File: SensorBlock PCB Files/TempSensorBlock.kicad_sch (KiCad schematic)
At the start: 11 parts, among them J1 Source Input (Screw), J2 Microcontroller Terminal (Scr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, U1 LM75B

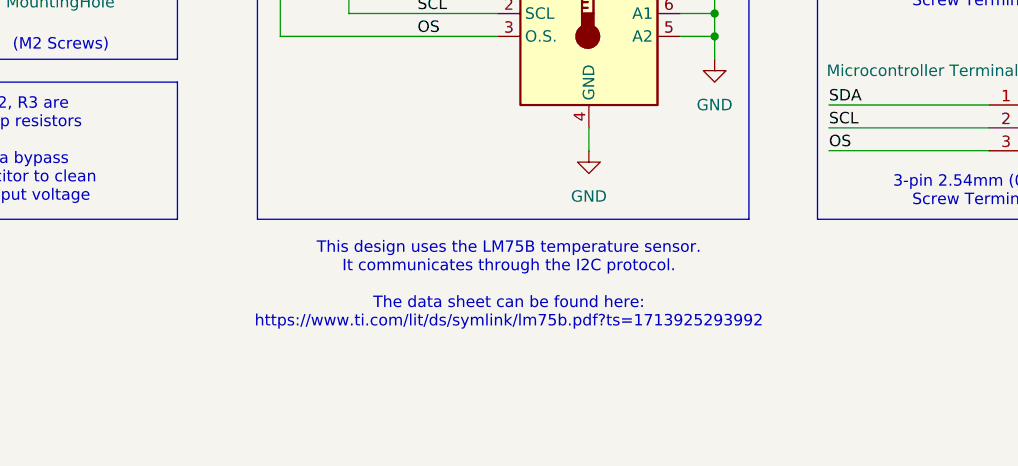
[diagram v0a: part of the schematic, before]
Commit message: Added documentation
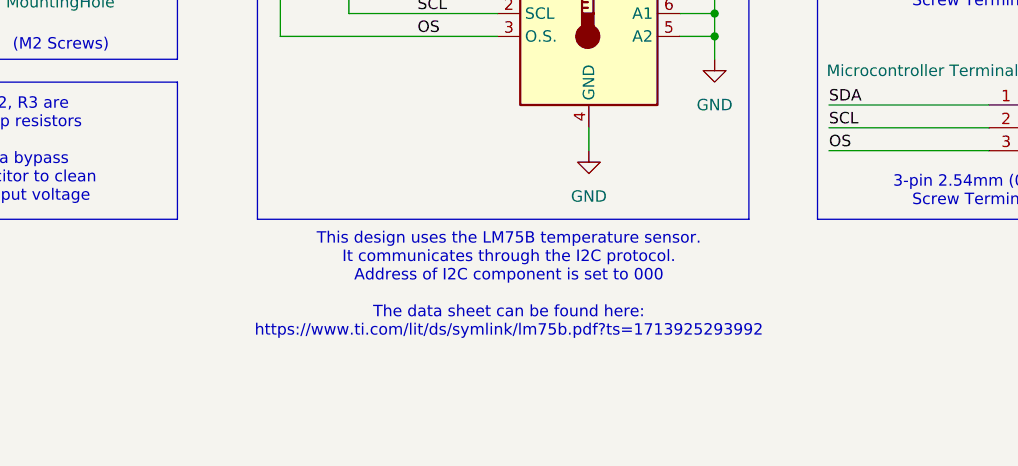
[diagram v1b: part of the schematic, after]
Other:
- note added: "This design uses the LM75B temperature sensor. It communicates through the I2C protocol. Address of I2C component is set to 000 The data sheet can be found here: https://www.ti.com/lit/ds/symlink/lm75b.pdf?ts=1713925293992"
- note removed: "This design uses the LM75B temperature sensor. It communicates through the I2C protocol. The data sheet can be found here: https://www.ti.com/lit/ds/symlink/lm75b.pdf?ts=1713925293992"
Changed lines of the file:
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@@
 		)
 	)
-	(text "This design uses the LM75B temperature sensor.\nIt communicates through the I2C protocol.\n\nThe data sheet can be found here:\nhttps://www.ti.com/lit/ds/symlink/lm75b.pdf?ts=1713925293992"
+	(text "This design uses the LM75B temperature sensor.\nIt communicates through the I2C protocol.\nAddress of I2C component is set to 000\n\nThe data sheet can be found here:\nhttps://www.ti.com/lit/ds/symlink/lm75b.pdf?ts=1713925293992"
 		(exclude_from_sim no)
 		(at 80.01 82.296 0)
